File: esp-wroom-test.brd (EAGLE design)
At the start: 44.4 x 38.9 mm, 26 parts, among them IC1 TCAN1051HGV, U1 NCP1117LPST50T3G, U2 XN04312, U8 NCP1117LPST50T3G

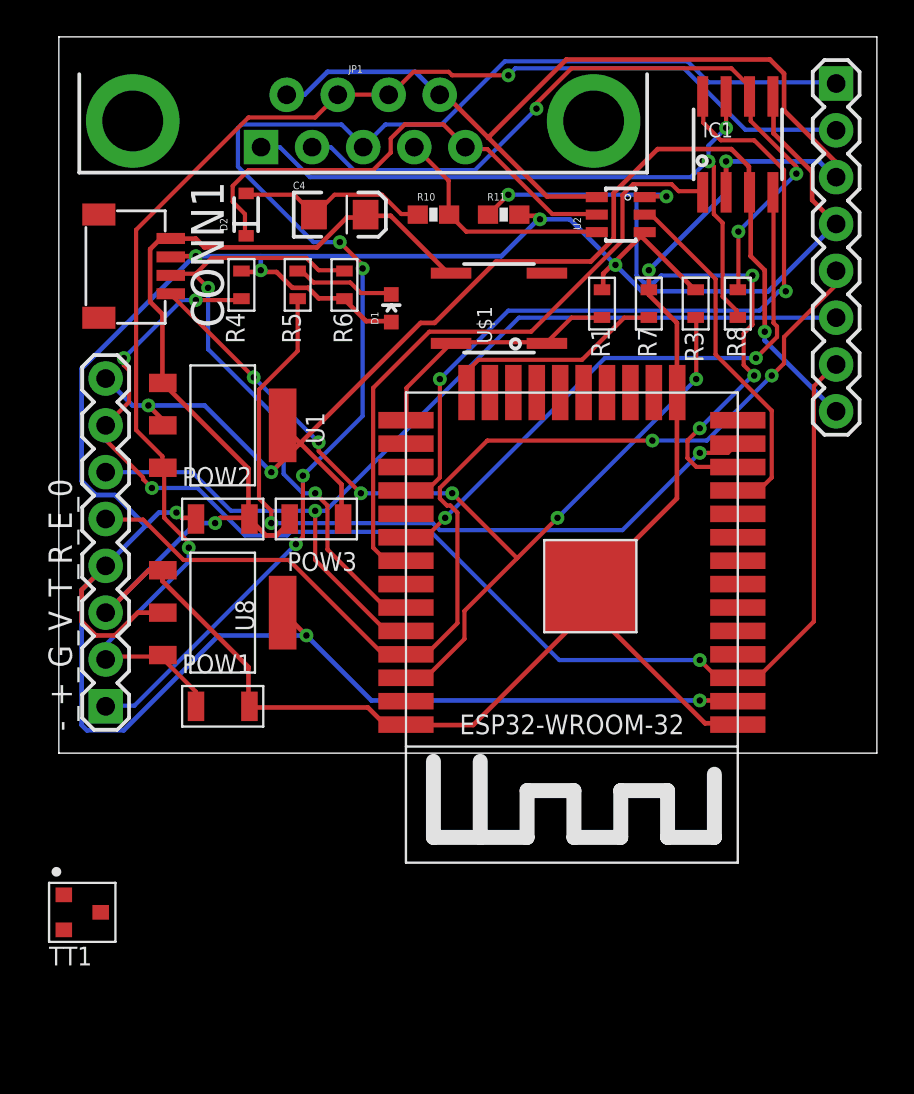
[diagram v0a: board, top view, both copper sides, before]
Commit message: Actually save
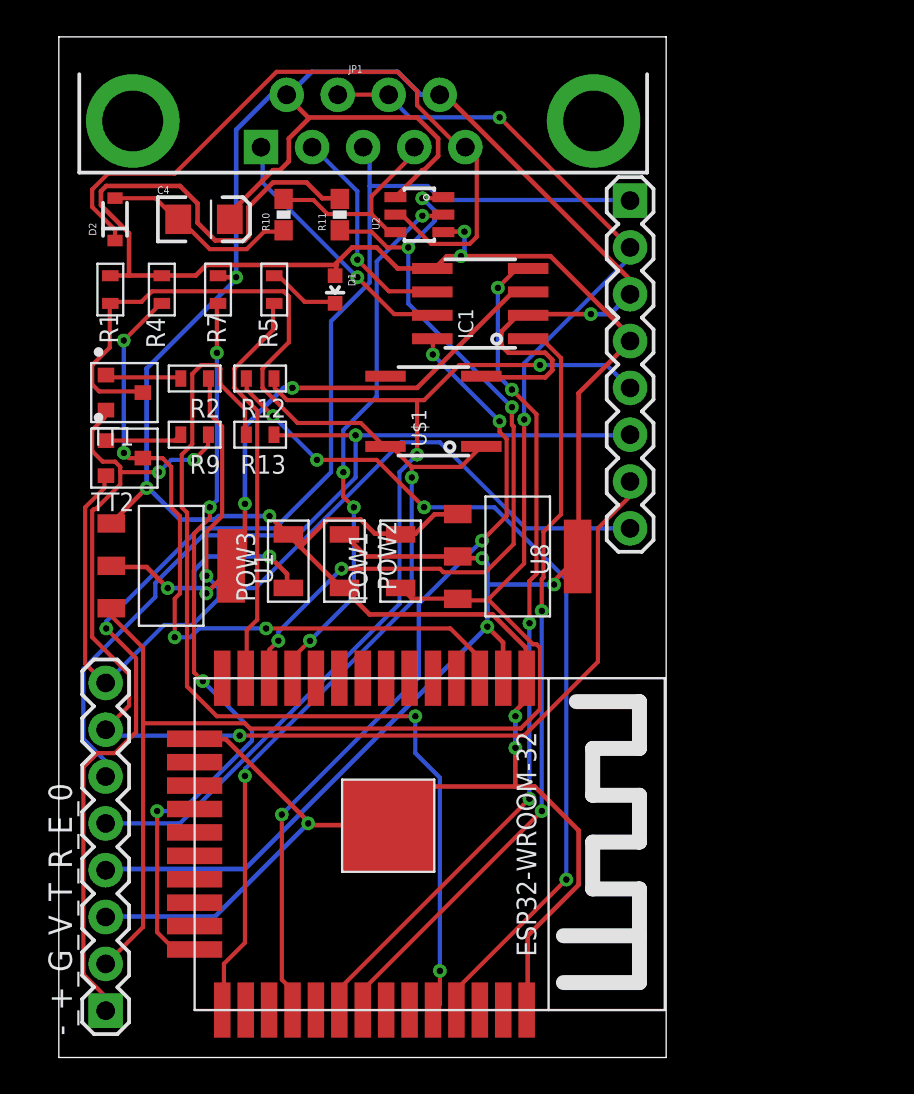
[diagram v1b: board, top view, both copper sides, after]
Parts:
- removed CONN1: STEMMA_I2C_QT, 01jim:JST_SH4
- removed R3, R6: (no value), 00jim:R0603
- removed R8: 200, 00jim:R0603
- added R12, R13, R2, R9: (no value), 00jim:R0603
- added TT2: MF-DSC-SOT233-MMBT3904, MF_Discrete_Semiconductor:SOT-23-3
- moved U$3 33.3 mm to (7.37, 4.06), turned to 270 degrees
- moved TT1 28.3 mm to (3.56, 19.6)
- moved R1 26.7 mm to (2.79, 25.1)
- moved R7 23.4 mm to (8.64, 25.1)
- moved -_+_G_V_T_R_E_0 16.5 mm to (2.54, -14.0)
- moved IC1 16.4 mm to (22.9, 24.4), turned to 90 degrees
- moved U8 16.3 mm to (24.9, 10.7)
- moved -_+_G_V_T_R_E_1 12.9 mm to (31.0, 30.0)
- moved POW1 12.5 mm to (18.5, 10.4), turned to 90 degrees
- moved U2 10.9 mm to (19.6, 29.2)
- moved R11 8.89 mm to (15.2, 29.2), turned to 90 degrees
- moved R10 8.13 mm to (12.2, 29.2), turned to 90 degrees
- moved U1 8.12 mm to (6.10, 10.2)
- moved C4 7.37 mm to (7.87, 29.0)
- moved D2 7.12 mm to (3.05, 29.0)
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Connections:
- removed net IO21_D1: TT1.P$3
- removed net N$1: TT1.P$2
- new net DTR: -_+_G_V_T_R_E_0.7, -_+_G_V_T_R_E_1.7, R9.P$1, TT1.P$2
- new net N$6: R9.P$2, TT2.P$1
- new net RTS: -_+_G_V_T_R_E_0.8, -_+_G_V_T_R_E_1.8, R2.P$1, TT2.P$2
- new net RXI_P: -_+_G_V_T_R_E_0.6, -_+_G_V_T_R_E_1.6, R13.P$1
- new net TXO_P: -_+_G_V_T_R_E_0.5, -_+_G_V_T_R_E_1.5, R12.P$1
- net CAN_H: no longer R8.P$1
- net CAN_L: no longer R8.P$2
- net EN: now also TT2.P$3; no longer -_+_G_V_T_R_E_0.7, -_+_G_V_T_R_E_1.7
- net GND: no longer CONN1.1
- net IO00: now also TT1.P$3
- net N$3: now also R2.P$2
- net RXI: now also R13.P$2; no longer -_+_G_V_T_R_E_0.6, -_+_G_V_T_R_E_1.6
- net SCL: no longer CONN1.4, R3.P$1
- net SDA: no longer CONN1.3, R6.P$1
- net TXO: now also R12.P$2; no longer -_+_G_V_T_R_E_0.5, -_+_G_V_T_R_E_1.5
- net VCC: no longer CONN1.2, R3.P$2, R6.P$2
- net VCC_50: no longer -_+_G_V_T_R_E_0.8, -_+_G_V_T_R_E_1.8
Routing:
- net DTR: track 0.00 -> 65.7 mm, vias 0 -> 3
- net RTS: track 0.00 -> 60.7 mm, vias 0 -> 1
- net IO00: track 14.0 -> 71.2 mm, vias 0 -> 2
- net TXO_P: track 0.00 -> 53.7 mm, vias 0 -> 2
- net SCL: track 51.7 -> 0.00 mm, vias 6 -> 0
- net RXI_P: track 0.00 -> 47.5 mm, vias 0 -> 1
- net VCC: track 153.1 -> 117.4 mm, vias 7 -> 5
- net SDA: track 34.0 -> 0.00 mm, vias 2 -> 0
- net EN: track 72.5 -> 40.0 mm
- net IO02: track 12.3 -> 41.3 mm, vias 0 -> 4
- net CAN_L: track 40.5 -> 11.9 mm, vias 3 -> 1
- net VCC_50: track 69.2 -> 41.7 mm, vias 3 -> 5
- net CAN_H: track 38.3 -> 14.2 mm, vias 2 -> 1
- net RAW: track 76.3 -> 96.8 mm
- net IO14: track 40.7 -> 22.0 mm, vias 2 -> 0
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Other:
- board size 44.4 x 38.9 mm -> 32.9 x 55.4 mm
